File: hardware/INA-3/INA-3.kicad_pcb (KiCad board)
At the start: 2 copper layers, 29.5 x 24.4 mm, 22 parts, among them J1 Conn_01x05, U1 OPA365, U2 OPA365, U3 OPA365, U4 AMS1117-1.8

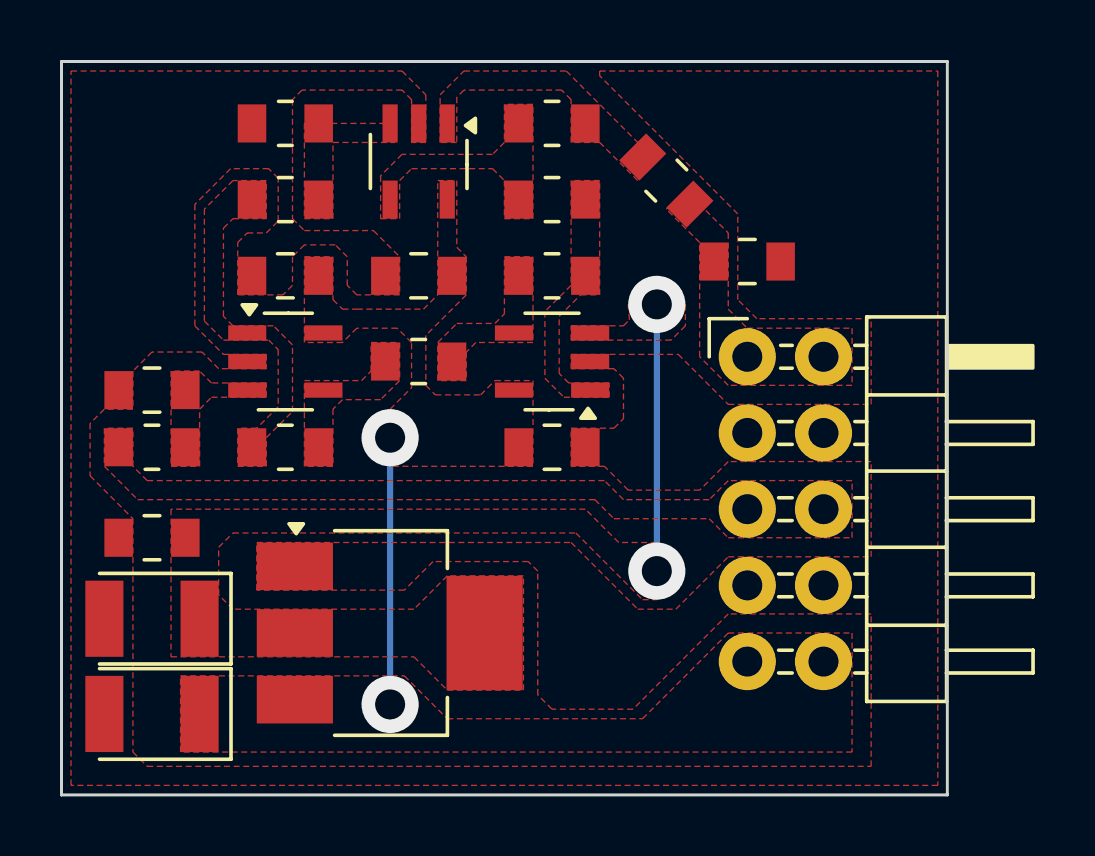
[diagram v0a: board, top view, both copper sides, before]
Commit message: modified:   firmware/ESU_V1/include/data_manager.h 	modified:   firmware/ESU_V1/include/hardware_control.h 	modified:   firmware/ESU_V1/src/hardware_control.cpp 	modified:   firmware/ESU_V1/src/main.cpp 	modified:   hardware/CTL-6.1/CTL-6.1.kicad_pcb 	modified:   hardware/CTL-6.1/CTL-6.1.kicad_prl 	modified:   hardware/CTL-6.1/CTL-6.1.kicad_pro 	modified:   hardware/INA-3/INA-3.kicad_pcb 	modified:   hardware/INA-3/INA-3.kicad_prl 	modified:   hardware/INA-3/INA-3.kicad_pro 	modified:   hardware/INA-3/INA-3.kicad_sch 	renamed:    hardware/INA-3/fabrication-outputs/INA-3-TRACE.dxf -> hardware/INA-3/fabrication-outputs/EDGE.dxf 	deleted:    hardware/INA-3/fabrication-outputs/INA-3-Edge_Cuts.dxf 	modified:   hardware/INA-3/fabrication-outputs/INA-3-F_Cu.dxf 	new file:   hardware/INA-3/fabrication-outputs/INA-3-F_Cu.pdf 	deleted:    hardware/INA-3/fabrication-outputs/INA-3-NPTH-drl_map.dxf 	deleted:    hardware/INA-3/fabrication-outputs/INA-3-PTH-drl_map.dxf 	new file:   hardware/INA-3/fabrication-outputs/TRACE.dxf 	deleted:    hardware/INA-3/fp-info-cache 	new file:   hardware/REM-5.0/.history 	modified:   hardware/REM-5.0/REM-5.0.kicad_pcb 	modified:   hardware/REM-5.0/REM-5.0.kicad_prl 	modified:   hardware/REM-5.0/REM-5.0.kicad_pro
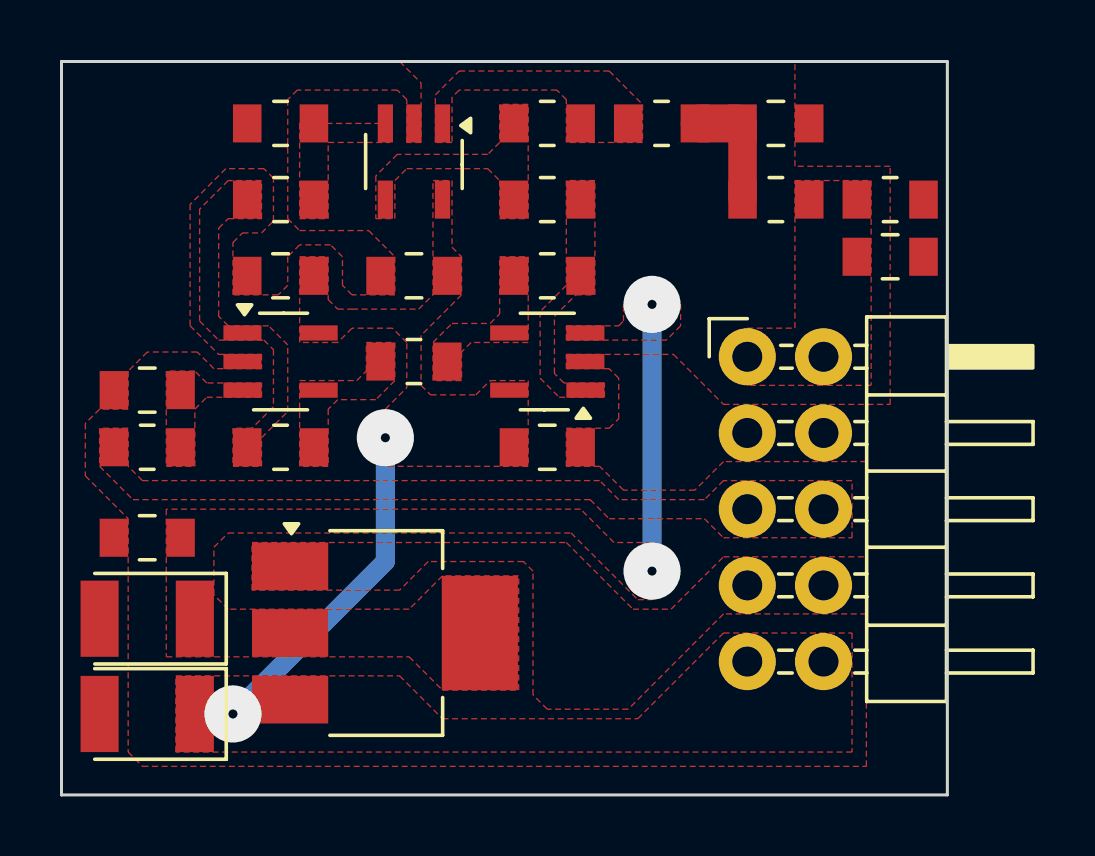
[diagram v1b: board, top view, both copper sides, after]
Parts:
- added C9: 100nF, Capacitor_SMD:C_0805_2012Metric_Pad1.18x1.45mm_HandSolder, F.Cu at (122.9, 57.3)
- added R10: 10kΩ, Resistor_SMD:R_0805_2012Metric_Pad1.20x1.40mm_HandSolder, F.Cu at (119.1, 55.4)
- added R11: 10kΩ, Resistor_SMD:R_0805_2012Metric_Pad1.20x1.40mm_HandSolder, F.Cu at (122.9, 55.4)
- moved C8 4.70 mm to (119.1, 52.9)
- moved R9 1.91 mm to (115.3, 52.9), turned to 0 degrees
- moved C1 0.16 mm to (102.6, 57.9)
- moved R3 0.16 mm to (102.6, 63.7)
- moved R5 0.16 mm to (102.6, 55.4)
- moved R7 0.16 mm to (102.6, 52.9)
- moved U2 0.16 mm to (102.6, 60.8)
- moved C2 0.16 mm to (111.4, 63.7)
- moved C3 0.16 mm to (107.0, 57.9)
- moved C4 0.16 mm to (98.1, 72.5)
- moved C5 0.16 mm to (98.1, 69.4)
- moved C6 0.16 mm to (98.1, 66.7)
- moved C7 0.16 mm to (98.1, 61.8)
- moved R1 0.16 mm to (107.0, 60.8)
- moved R2 0.16 mm to (111.4, 57.9)
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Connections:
- C8 pad 1: /OUT -> Net-(C8-Pad1)
- R9 pad 2: /OUT -> Net-(C8-Pad1)
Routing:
- net Net-(C8-Pad1): track 0.00 -> 3.81 mm
- net +5V: track 8.41 -> 11.3 mm

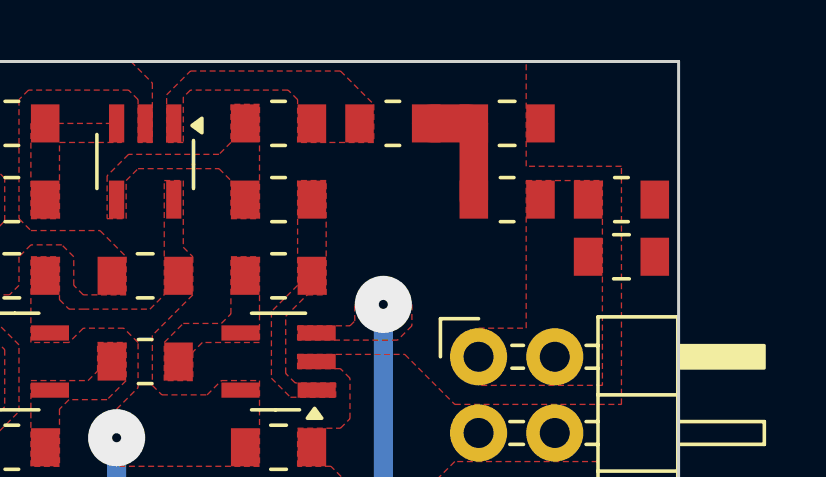
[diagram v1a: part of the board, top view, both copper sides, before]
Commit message: new file:   hardware/INA-3/.history 	modified:   hardware/INA-3/INA-3.kicad_pcb 	modified:   hardware/INA-3/INA-3.kicad_prl 	modified:   hardware/INA-3/INA-3.kicad_pro 	modified:   hardware/INA-3/fabrication-outputs/EDGE.dxf 	modified:   hardware/INA-3/fabrication-outputs/TRACE.dxf 	new file:   hardware/INA-3/~INA-3.kicad_pcb.lck 	new file:   hardware/INA-3/~INA-3.kicad_pro.lck
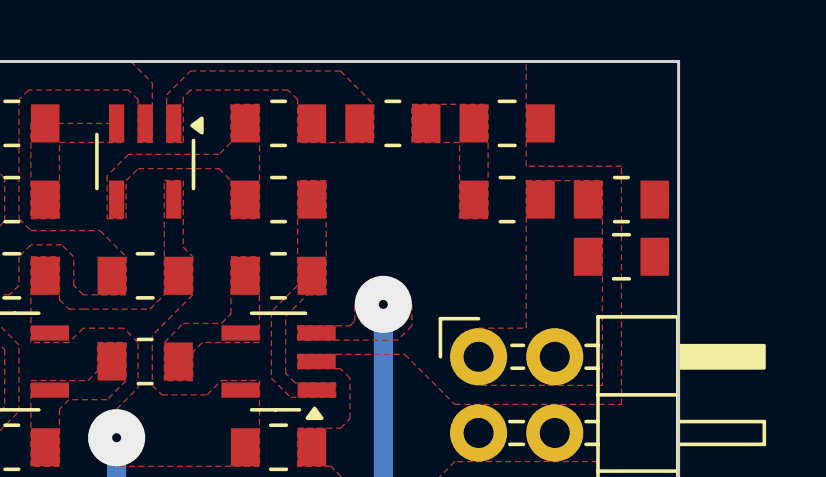
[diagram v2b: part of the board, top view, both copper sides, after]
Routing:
- net Net-(C8-Pad1): track 3.81 -> 0.00 mm
- added copper zone on F.Cu, net Net-(C8-Pad1)
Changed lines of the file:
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@@
 		(layer "Edge.Cuts")
-	)
-	(segment
-		(start 117.95125 52.86375)
-		(end 117.95125 55.40375)
-		(width 0.9525)
-		(layer "F.Cu")
-		(net "Net-(C8-Pad1)")
-	)
-	(segment
-		(start 116.5225 52.86375)
-		(end 117.7925 52.86375)
-		(width 1.27)
-		(layer "F.Cu")
-		(net "Net-(C8-Pad1)")
 	)
 	(via
@@
 			)
 		)
+	)
+	(zone
+		(net "Net-(C8-Pad1)")
+		(layer "F.Cu")
+		(hatch none 0.5)
+		(priority 1)
+		(connect_pads yes
+			(clearance 0)
+		)
+		(min_thickness 0.03175)
+		(fill yes
+			(thermal_gap 0.5)
+			(thermal_bridge_width 0.5)
+			(island_removal_mode 0)
+		)
+		(polygon
+			(pts
+				(xy 115.8875 52.22875) (xy 118.4275 52.22875) (xy 118.4275 56.03875) (xy 117.475 56.03875) (xy 117.475 53.49875)
+				(xy 115.8875 53.49875)
+			)
+		)
